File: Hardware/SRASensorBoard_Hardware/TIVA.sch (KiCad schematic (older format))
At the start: 7 parts, among them U4 TM4C129E_Launchpad

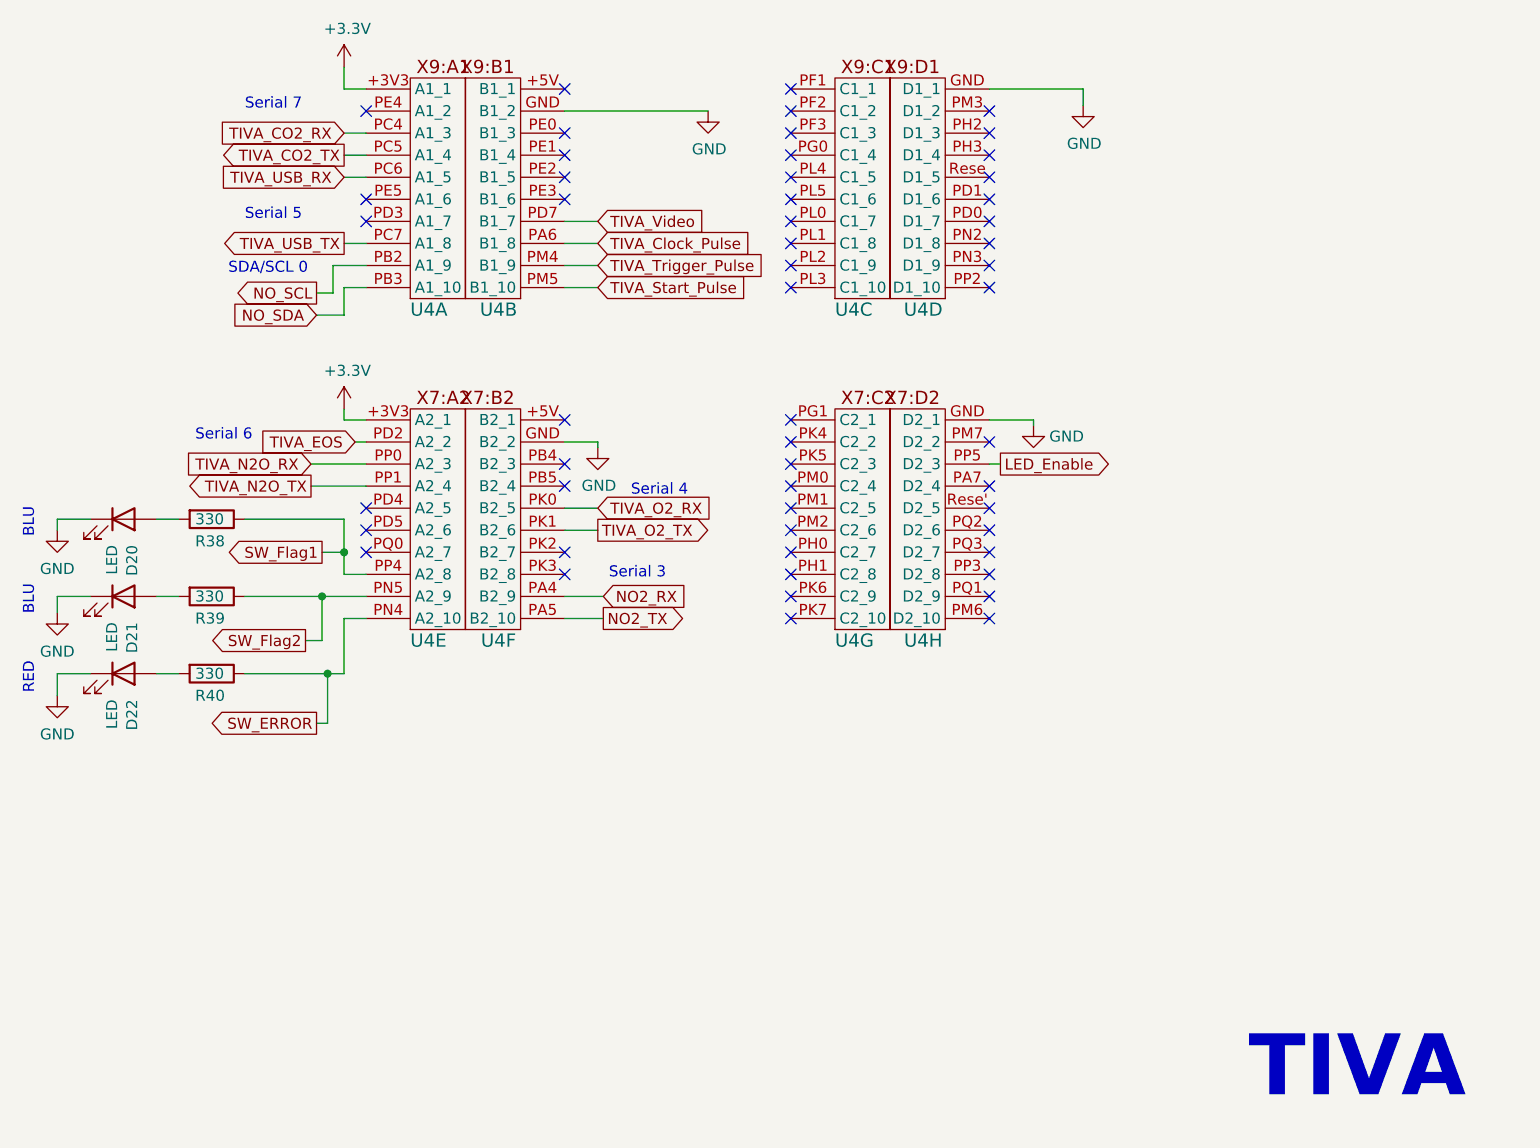
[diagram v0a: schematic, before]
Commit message: Board Progress 7 (final rev 1)
Final edits for REV 1
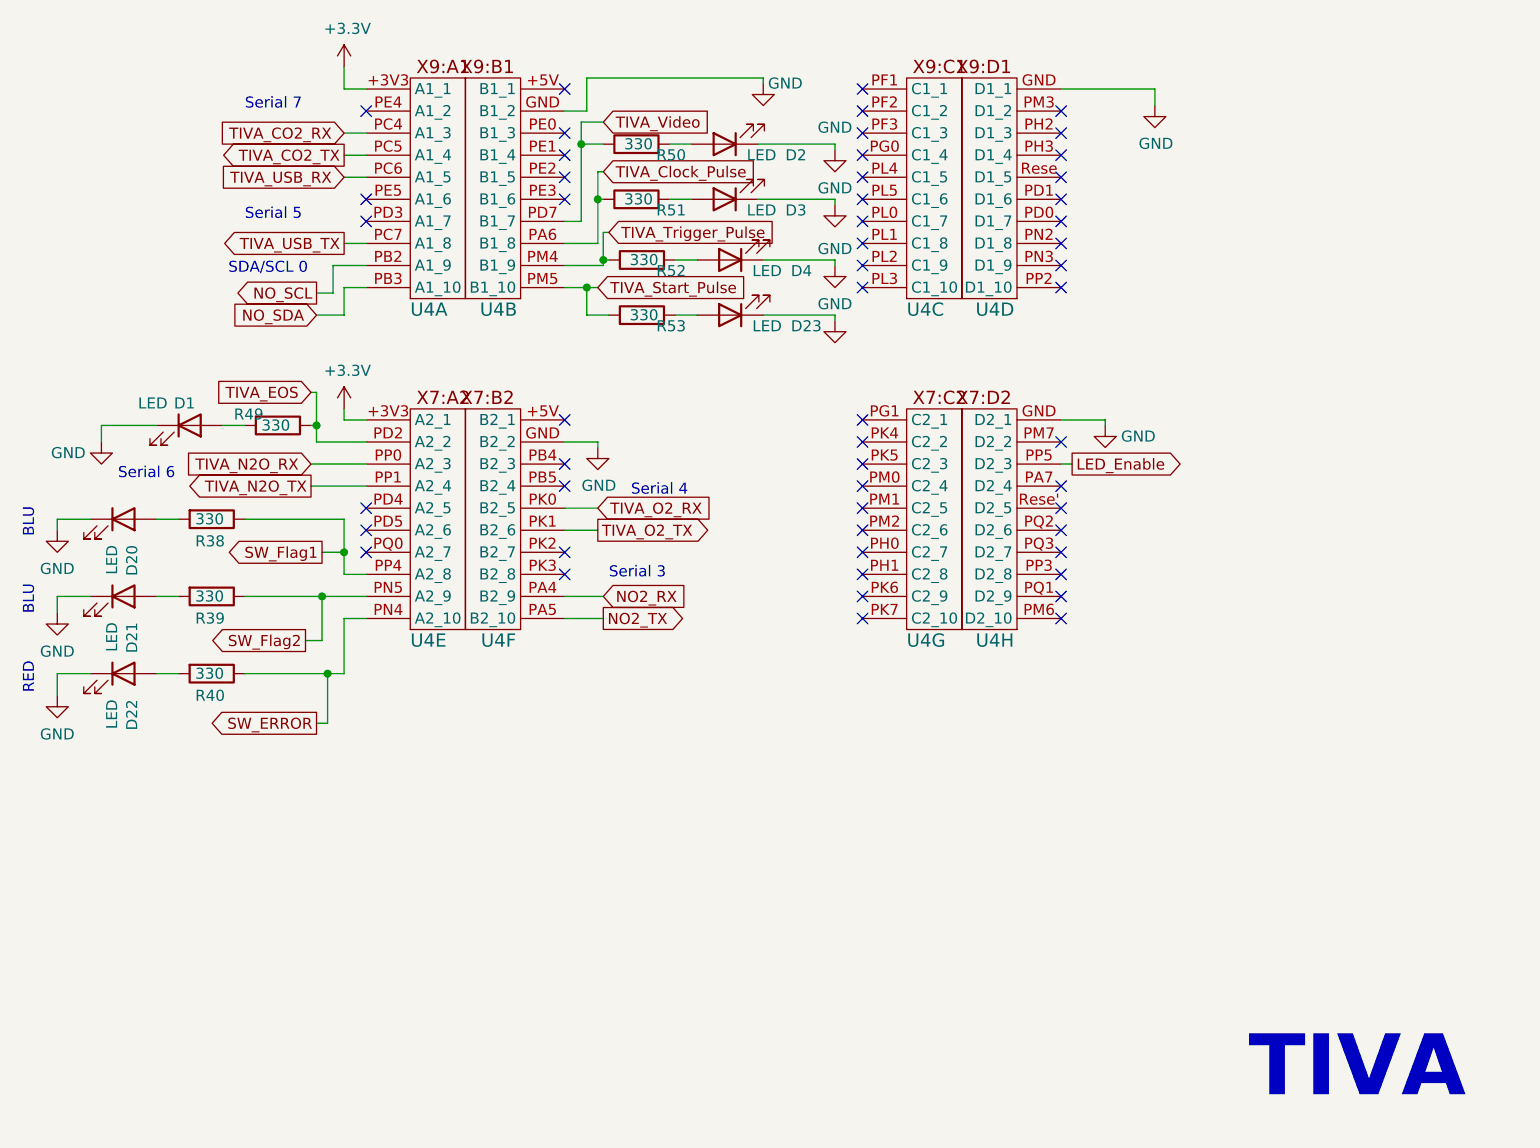
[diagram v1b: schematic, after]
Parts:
- added D1, D2, D23, D3, D4: LED, Diode_SMD:D_0603_1608Metric_Pad1.05x0.95mm_HandSolder, symbol Device:LED
- added R49, R50, R51, R52, R53: 330, Resistor_SMD:R_0603_1608Metric_Pad1.05x0.95mm_HandSolder, symbol Device:R
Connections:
- net GND: now also D1.1 (K), D2.1 (K), D23.1 (K), D3.1 (K), D4.1 (K)
- net TIVA_Clock_Pulse: now also R51.1
- net TIVA_EOS: now also R49.1
- net TIVA_Start_Pulse: now also R53.1
- net TIVA_Trigger_Pulse: now also R52.1
- net TIVA_Video: now also R50.1
- new net: D2.2 (A), R50.2
- new net: D3.2 (A), R51.2
- new net: D4.2 (A), R52.2
- new net: D23.2 (A), R53.2
- new net: D1.2 (A), R49.2
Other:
- moved on the sheet: U4C, U4D, U4G, U4H
